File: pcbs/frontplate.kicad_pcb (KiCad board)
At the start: 2 copper layers, 129.8 x 107.9 mm, 5 parts

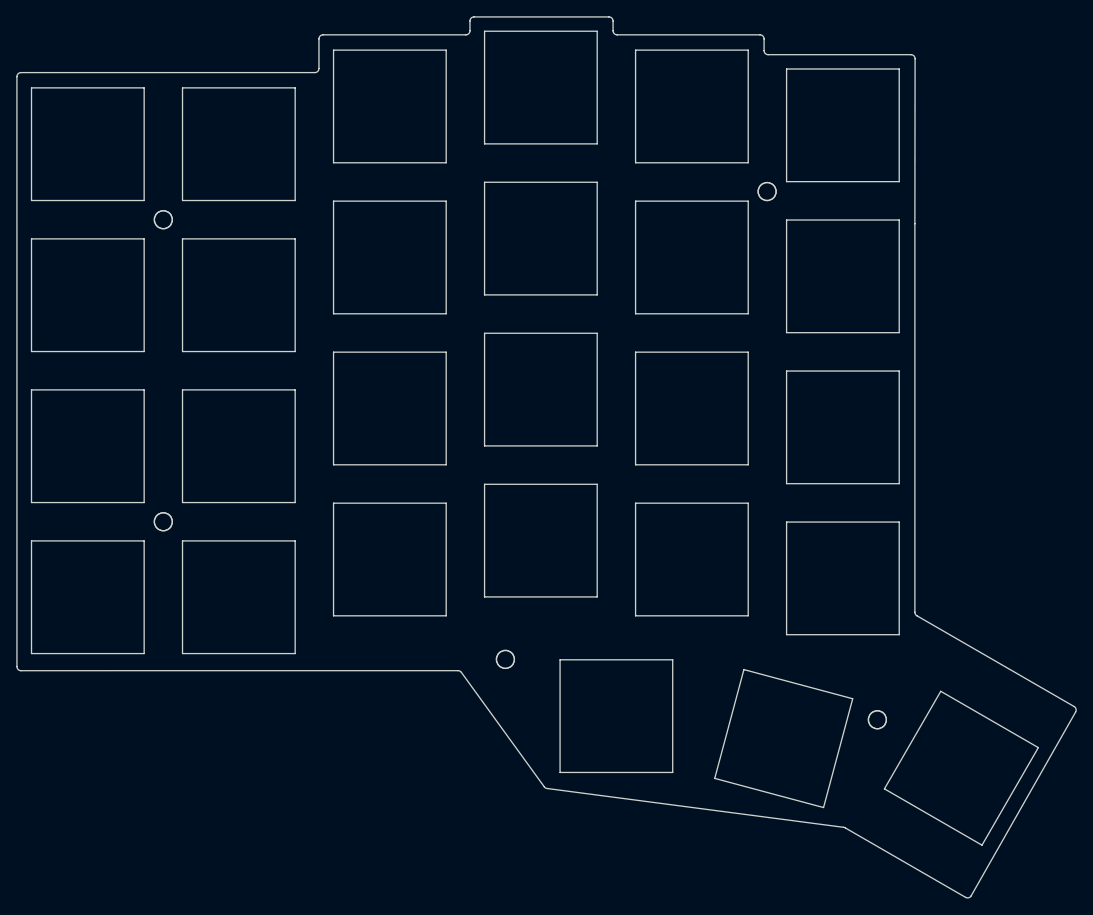
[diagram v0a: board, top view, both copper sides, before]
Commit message: Archive ordered wireless PCB and manufacturing files
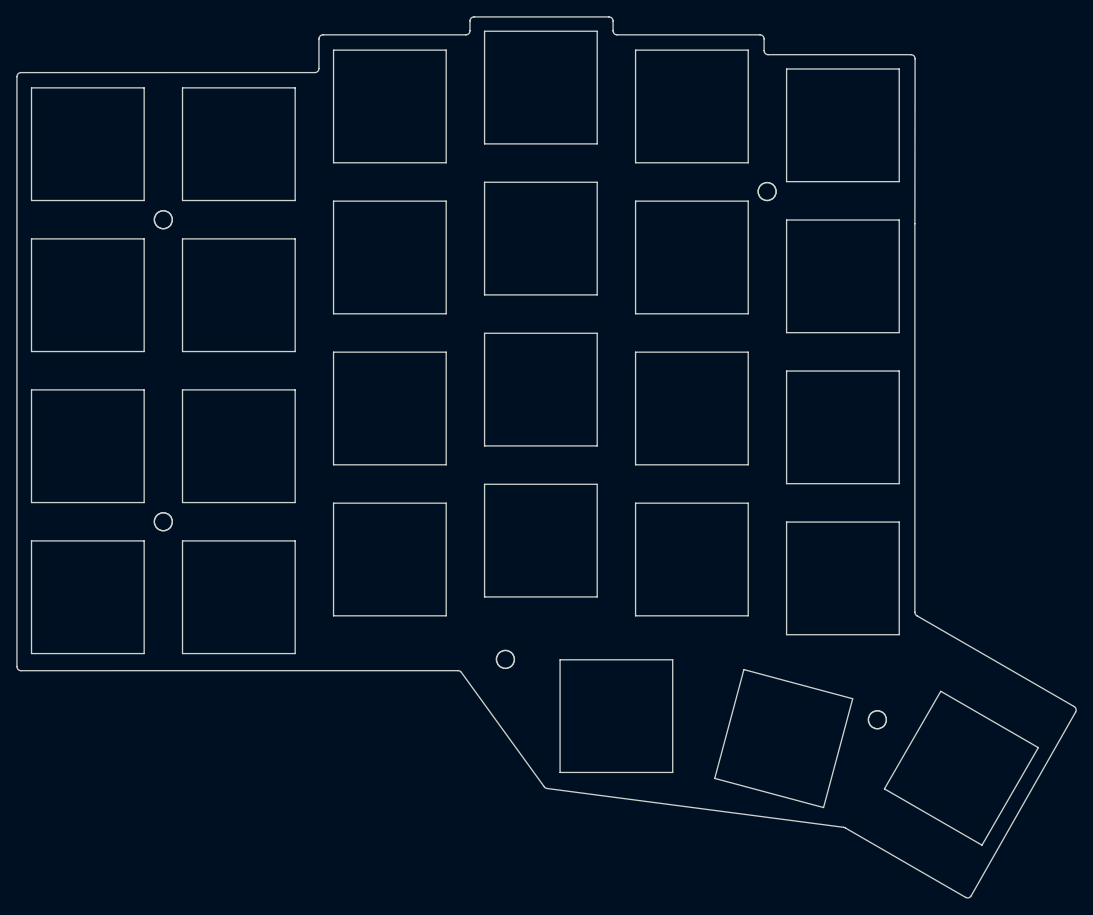
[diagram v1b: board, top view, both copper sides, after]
